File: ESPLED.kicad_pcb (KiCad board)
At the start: 2 copper layers, 81.3 x 83.8 mm, 24 parts, among them CON1 BARREL_JACK, J1 USB_B_Micro, P2 LED_CON, P3 LED_CON_SCREW, P4 LED_CON_SCREW, Q1 IRLZ34N, Q2 IRLZ34N, Q3 IRLZ34N, SW1 Reset, SW2 Program, U1 LM1117-3.3, U2 ESP-07v2, U3 INTERFACE-CH340G, Y1 Crystal

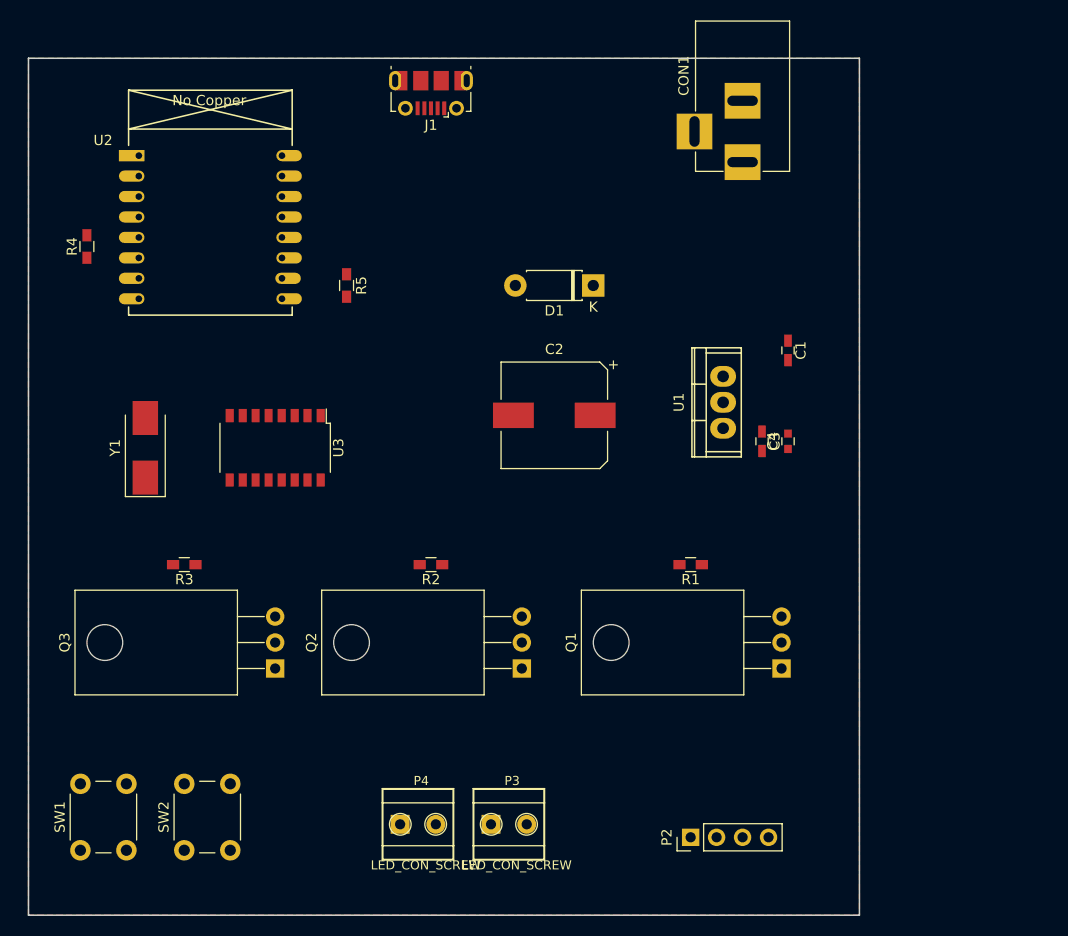
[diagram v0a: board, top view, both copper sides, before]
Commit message: Footprint research done, layout more or less gelayoutet
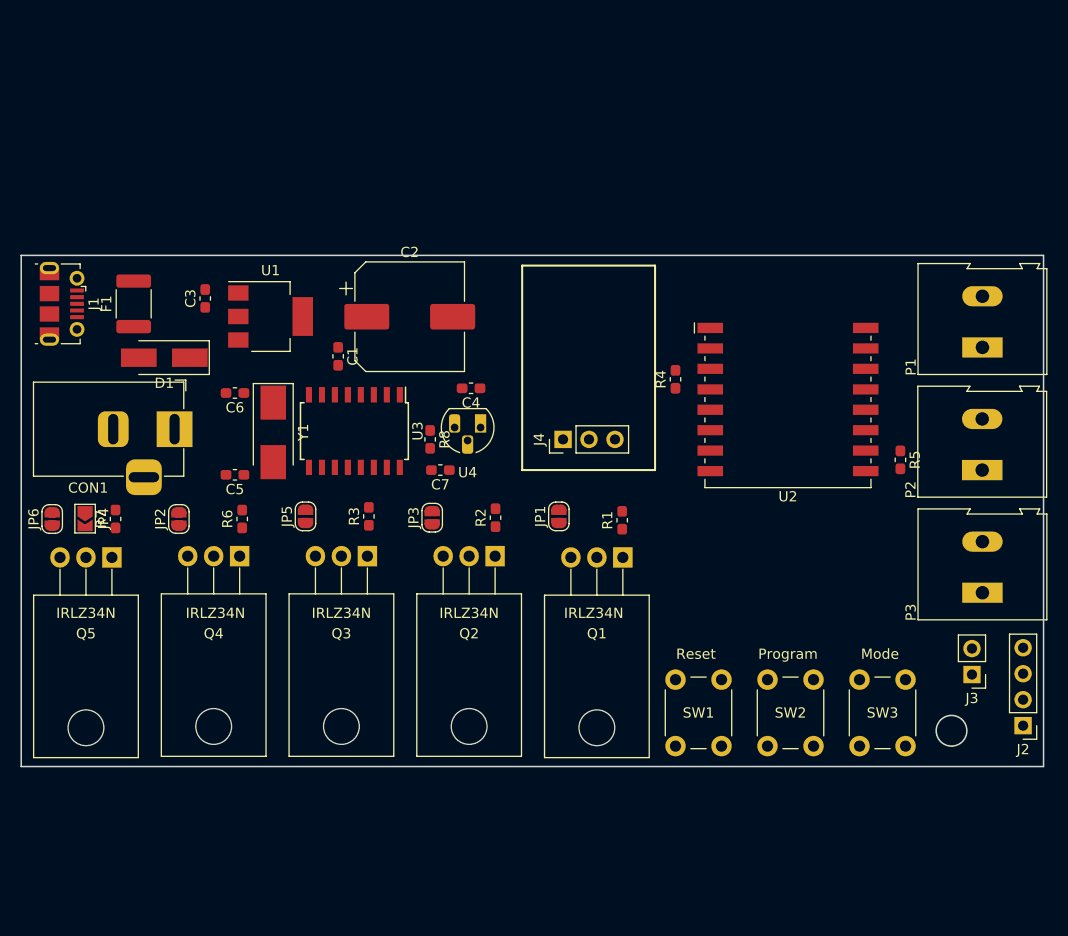
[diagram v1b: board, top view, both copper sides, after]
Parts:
- removed P4: LED_CON_SCREW, SeeedOPL-Connector:H2-3.5-7.0X7.0MM
- added C5: 22p, Capacitor_SMD:C_0603_1608Metric_Pad1.05x0.95mm_HandSolder, F.Cu at (112.9, 86.5)
- added C6: 22p, Capacitor_SMD:C_0603_1608Metric_Pad1.05x0.95mm_HandSolder, F.Cu at (112.9, 78.5)
- added C7: 100n, Capacitor_SMD:C_0603_1608Metric_Pad1.05x0.95mm_HandSolder, F.Cu at (133.0, 86.0)
- added F1: Polyfuse, Fuse:Fuse_1812_4532Metric_Pad1.30x3.40mm_HandSolder, F.Cu at (103.0, 69.7)
- added J2: LED_CON_RGB, Connector_PinHeader_2.54mm:PinHeader_1x04_P2.54mm_Vertical, F.Cu at (190.0, 111.0)
- added J3: LED_CON_WW, Connector_PinHeader_2.54mm:PinHeader_1x02_P2.54mm_Vertical, F.Cu at (185.0, 106.0)
- added J4: MIC, Connector_PinHeader_2.54mm:PinHeader_1x03_P2.54mm_Vertical, F.Cu at (145.0, 83.0)
- added JP1: GPIO LINK, Jumper:SolderJumper-2_P1.3mm_Open_RoundedPad1.0x1.5mm, F.Cu at (144.6, 90.5)
- added JP2: GPIO LINK, Jumper:SolderJumper-2_P1.3mm_Open_RoundedPad1.0x1.5mm, F.Cu at (107.4, 90.8)
- added JP3: GPIO LINK, Jumper:SolderJumper-2_P1.3mm_Open_RoundedPad1.0x1.5mm, F.Cu at (132.2, 90.7)
- added JP4: GND LINK, Jumper:SolderJumper-2_P1.3mm_Open_TrianglePad1.0x1.5mm, F.Cu at (98.2, 90.8)
- added JP5: GPIO LINK, Jumper:SolderJumper-2_P1.3mm_Open_RoundedPad1.0x1.5mm, F.Cu at (119.8, 90.5)
- added JP6: GPIO LINK, Jumper:SolderJumper-2_P1.3mm_Open_RoundedPad1.0x1.5mm, F.Cu at (95.0, 90.8)
- added P1: LED_CON_SCREW, TerminalBlock:TerminalBlock_Altech_AK300-2_P5.00mm, F.Cu at (186.0, 74.0)
- added Q4: IRLZ34N, Package_TO_SOT_THT:TO-220-3_Horizontal_TabDown, F.Cu at (113.4, 94.4)
- added Q5: IRLZ34N, Package_TO_SOT_THT:TO-220-3_Horizontal_TabDown, F.Cu at (100.9, 94.5)
- added R6: 100, Resistor_SMD:R_0603_1608Metric_Pad1.05x0.95mm_HandSolder, F.Cu at (113.6, 90.8)
- added R7: 100, Resistor_SMD:R_0603_1608Metric_Pad1.05x0.95mm_HandSolder, F.Cu at (101.2, 90.8)
- added R8: 4.7K, Resistor_SMD:R_0603_1608Metric_Pad1.05x0.95mm_HandSolder, F.Cu at (132.0, 83.0)
- added SW3: Mode, Button_Switch_THT:SW_PUSH_6mm, F.Cu at (174.0, 113.0)
- added U4: DS18B20, Package_TO_SOT_THT:TO-92_HandSolder, F.Cu at (136.9, 81.8)
- C1, C3: footprint Capacitors_SMD:C_0603_HandSoldering -> Capacitor_SMD:C_0603_1608Metric_Pad1.05x0.95mm_HandSolder
- C2: footprint Capacitors_SMD:CP_Elec_10x10.5 -> Capacitor_SMD:CP_Elec_10x10.5
- C4: footprint Capacitors_SMD:C_0603 -> Capacitor_SMD:C_0603_1608Metric_Pad1.05x0.95mm_HandSolder
- CON1: footprint Connectors:BARREL_JACK -> Connector_BarrelJack:BarrelJack_Horizontal
- D1: value 1N5819 -> 1N5817; footprint Diode_THT:D_DO-41_SOD81_P7.62mm_Horizontal -> Diode_SMD:D_SMA_Handsoldering
- J1: footprint Connectors_USB:USB_Micro-B_Molex-105017-0001 -> Connector_USB:USB_Micro-B_Molex-105017-0001
- P2: value LED_CON -> LED_CON_SCREW; footprint Pin_Headers:Pin_Header_Straight_1x04_Pitch2.54mm -> TerminalBlock:TerminalBlock_Altech_AK300-2_P5.00mm
- P3: footprint SeeedOPL-Connector:H2-3.5-7.0X7.0MM -> TerminalBlock:TerminalBlock_Altech_AK300-2_P5.00mm
- Q1, Q2, Q3: footprint TO_SOT_Packages_THT:TO-220_Horizontal -> Package_TO_SOT_THT:TO-220-3_Horizontal_TabDown
- R1, R2, R3, R4, R5: footprint Resistors_SMD:R_0603_HandSoldering -> Resistor_SMD:R_0603_1608Metric_Pad1.05x0.95mm_HandSolder
- SW1: footprint Buttons_Switches_THT:SW_PUSH_6mm_h5mm -> Button_Switch_THT:SW_PUSH_6mm
- SW2: footprint Button_Switch_THT:SW_PUSH_6mm_H5mm -> Button_Switch_THT:SW_PUSH_6mm
- U1: value LM1117-3.3 -> AMS1117-3.3; footprint Power_Integrations:TO-220 -> Package_TO_SOT_SMD:SOT-223-3_TabPin2
- U2: footprint ESP8266:ESP-07v2 -> RF_Module:ESP-07
- U3: footprint Housings_SSOP:SOP-16_4.4x10.4mm_Pitch1.27mm -> Package_SO:SOIC-16W_5.3x10.2mm_P1.27mm
- moved U2 67.1 mm to (167.0, 77.0)
- moved CON1 61.4 mm to (107.0, 82.0), turned to 0 degrees
- moved SW1 59.1 mm to (156.0, 113.0)
- moved R4 59.0 mm to (156.0, 77.1)
- moved SW2 58.0 mm to (165.0, 113.0)
- moved R5 56.8 mm to (178.0, 85.0)
- moved C3 56.2 mm to (110.0, 69.2), turned to 90 degrees
- moved P3 51.6 mm to (186.0, 98.0), turned to 90 degrees
- moved P2 45.9 mm to (186.0, 86.0)
- moved U1 45.1 mm to (116.4, 71.0), turned to 0 degrees
- moved C1 44.0 mm to (123.0, 74.9)
- moved D1 42.5 mm to (106.0, 75.0)
- moved J1 42.0 mm to (96.0, 69.7), turned to 270 degrees
- moved C4 31.4 mm to (136.0, 78.0), turned to 180 degrees
- moved Q1 18.9 mm to (150.8, 94.5), turned to 180 degrees
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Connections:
- D1 pad 2: VUSB -> Net-(D1-Pad2)
- P2 pad 1: Net-(P2-Pad1) -> Net-(J2-Pad1)
- P2 pad 2: Net-(P2-Pad2) -> Net-(J2-Pad2)
- P3 pad 1: Net-(P2-Pad3) -> Net-(J3-Pad1)
- P3 pad 2: +12V -> Net-(J3-Pad2)
- Q1 pad 2: Net-(P2-Pad1) -> Net-(J2-Pad3)
- Q2 pad 2: Net-(P2-Pad2) -> Net-(J2-Pad1)
- Q3 pad 2: Net-(P2-Pad3) -> Net-(J3-Pad1)
- R1 pad 2: Net-(R1-Pad2) -> Net-(JP1-Pad2)
- R2 pad 2: Net-(R2-Pad2) -> Net-(JP3-Pad2)
- R3 pad 2: Net-(R3-Pad2) -> Net-(JP5-Pad2)
- U2 pad 4: Net-(U2-Pad4) -> Net-(JP5-Pad2)
- U2 pad 5: Net-(R3-Pad2) -> Net-(JP3-Pad2)
- U2 pad 6: Net-(R2-Pad2) -> Net-(JP1-Pad2)
- U2 pad 7: Net-(R1-Pad2) -> Net-(JP2-Pad2)
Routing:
- removed copper zone on F.Cu, net GND
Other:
- board size 81.3 x 83.8 mm -> 100 x 50 mm
